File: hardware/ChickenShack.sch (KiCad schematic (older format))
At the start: 44 parts, among them P1 BATTERY, P2 SPARE, P3 SCOPE, P4 DEBUG, P5 D_MOTOR, P6 LIGHT, P7 D_SENSOR, P8 D_SWITCH, Q1 MOSFET_N, Q2 MOSFET_P, U1 MCP1702, U2 ATMEGA88-AU, X1 CRYSTAL

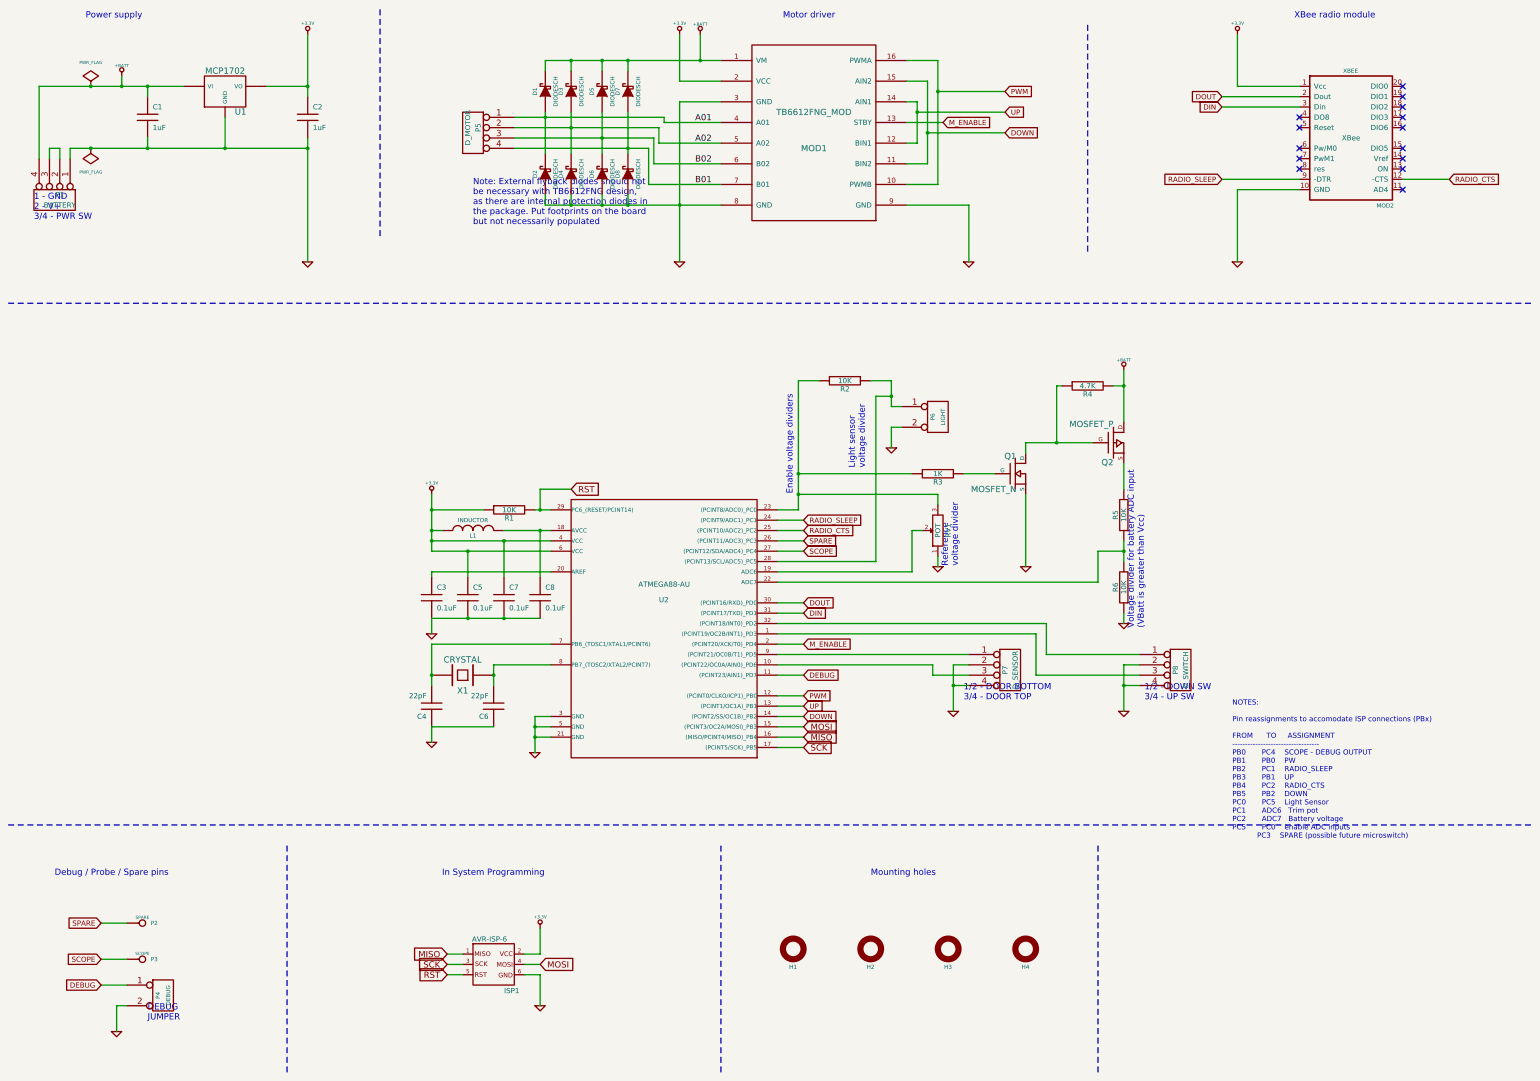
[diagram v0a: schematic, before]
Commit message: More layout
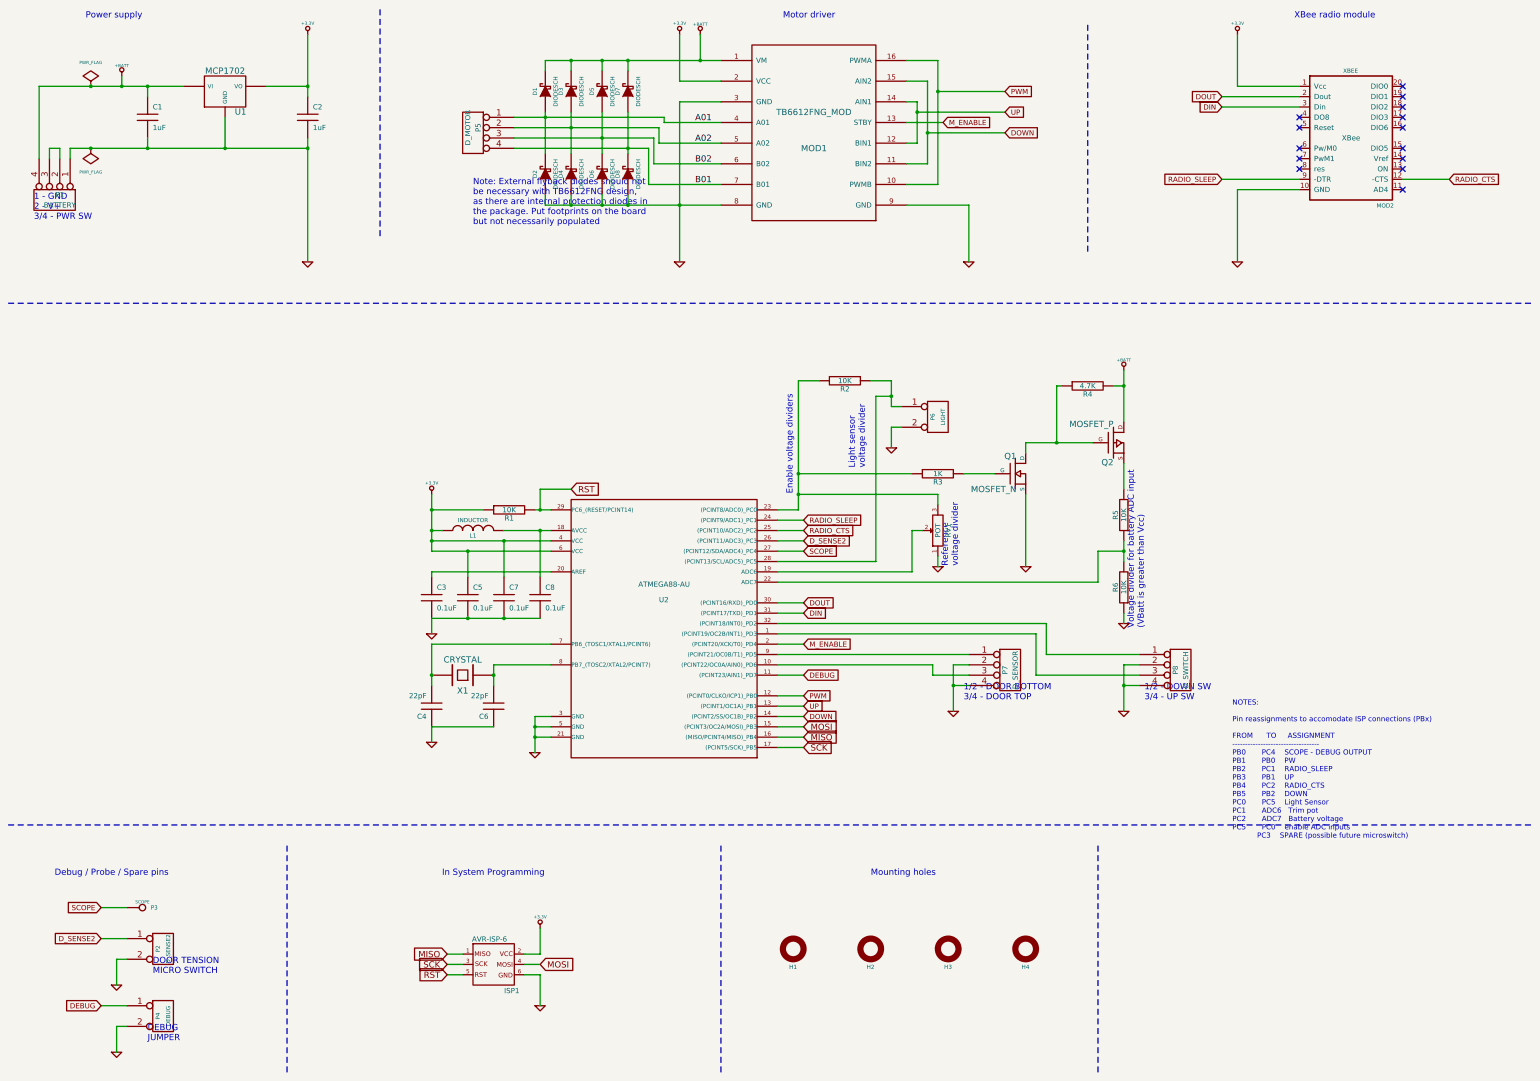
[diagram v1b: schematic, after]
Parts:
- removed P2: SPARE, symbol CONN_1
- added P2: D_SENSE2, symbol CONN_2
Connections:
- net GND: now also P2.2 (PM)
- net SPARE renamed D_SENSE2
- net D_SENSE2: now also P2.1 (P1)
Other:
- note added: "DOOR TENSION\nMICRO SWITCH"
- moved on the sheet: P3, P4
